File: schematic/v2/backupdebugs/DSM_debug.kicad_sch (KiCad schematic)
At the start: 16 parts, among them J16 DSM_DBG, J20 USB_A, U33 CH340G, Y2 Crystal

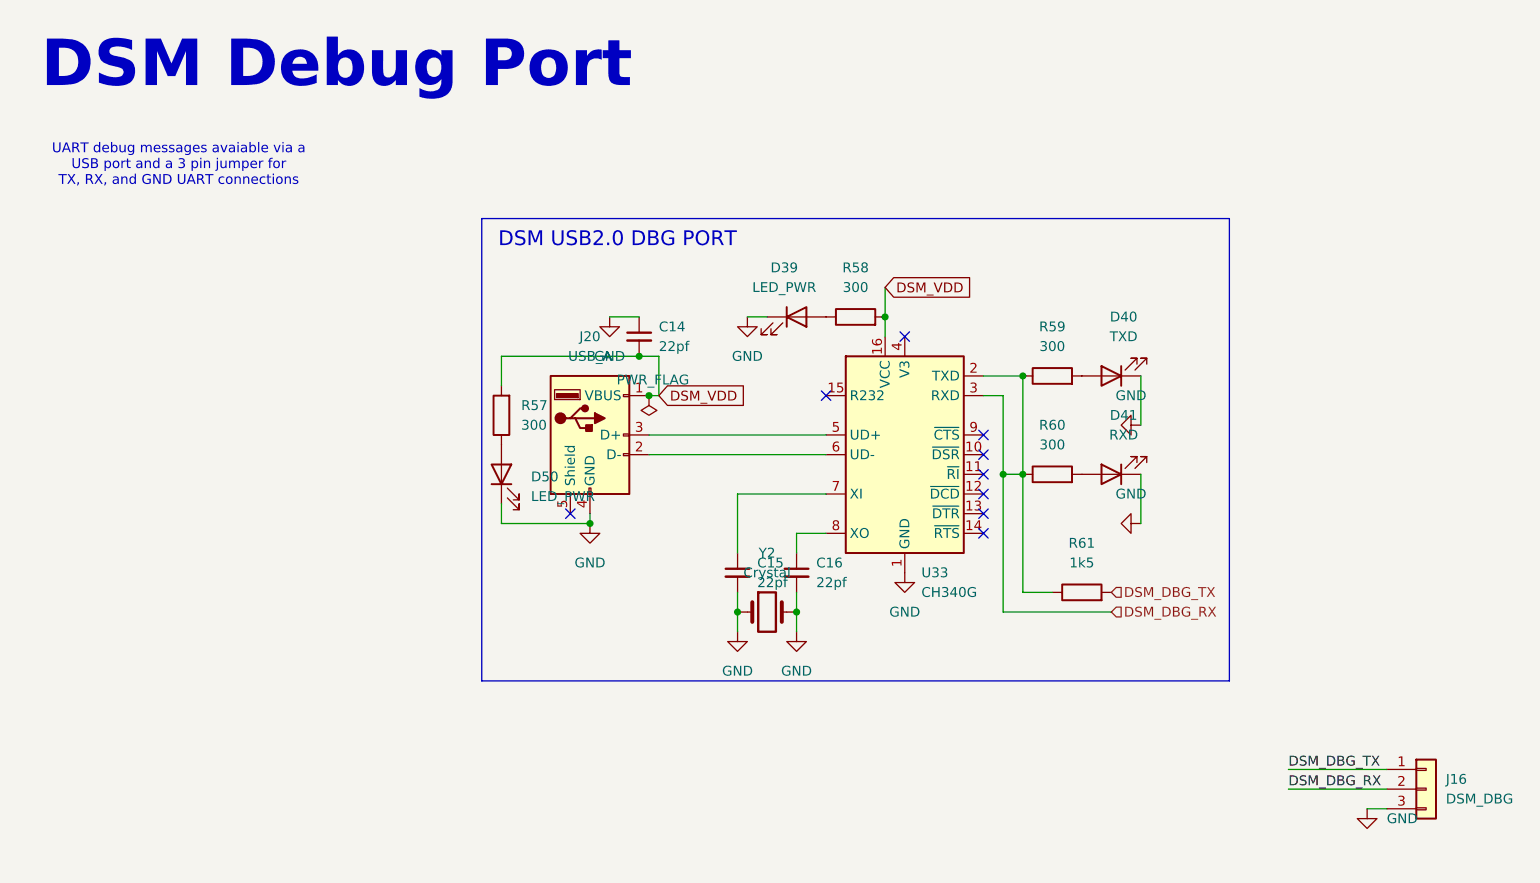
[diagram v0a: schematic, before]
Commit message: time to start routing?
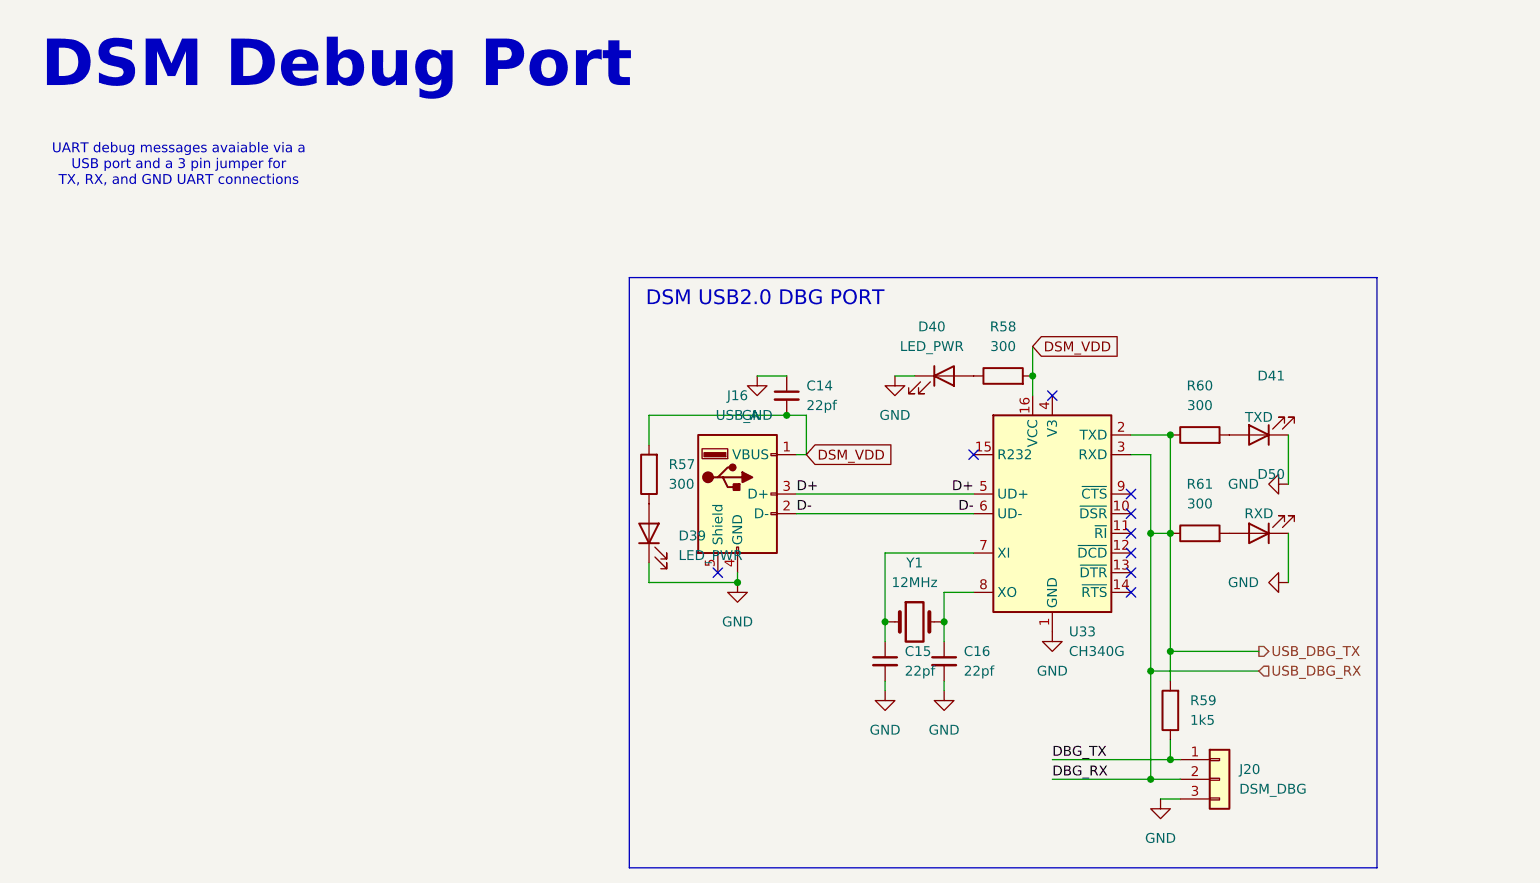
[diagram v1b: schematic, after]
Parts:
- removed J16: DSM_DBG, Connector_PinHeader_1.00mm:PinHeader_1x03_P1.00mm_Horizontal, symbol Connector_Generic:Conn_01x03
- removed J20: USB_A, Connector_USB:USB_A_CNCTech_1001-011-01101_Horizontal, symbol Connector:USB_A
- removed Y2: Crystal, symbol Device:Crystal
- added J16: USB_A, Connector_USB:USB_A_CNCTech_1001-011-01101_Horizontal, symbol Connector:USB_A
- added J20: DSM_DBG, Connector_PinHeader_1.00mm:PinHeader_1x03_P1.00mm_Horizontal, symbol Connector_Generic:Conn_01x03
- added Y1: 12MHz, Crystal:Crystal_HC49-4H_Vertical, symbol Device:Crystal
- D40: value TXD -> LED_PWR
- D41: value RXD -> TXD
- D50: value LED_PWR -> RXD
- R59: value 300 -> 1k5
- R61: value 1k5 -> 300
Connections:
- net DSM_VDD: now also J16.1 (VBUS)
- net GND: now also J16.4 (GND), J20.3 (Pin_3)
- net at R57.1: now also D39.2 (A); no longer D50.2 (A)
- net D+: now reaches U33.5 (UD+)
- net D+: now also J16.3 (D+)
- net D-: now reaches U33.6 (UD-)
- net D-: now also J16.2 (D-)
- net at C15.1, U33.7 (XI): now also Y1.1
- net at C16.1, U33.8 (XO): now also Y1.2
- net at D40.2 (A): now also R58.1; no longer R59.2
- net DSM_DBG_RX renamed USB_DBG_RX
- net USB_DBG_RX: now also R59.2, J20.2 (Pin_2); no longer R59.1
- net DSM_DBG_TX: no longer names the net of R61.2
- net DSM_DBG_TX: now also D50.2 (A)
- new net DBG_TX: J20.1 (Pin_1), R59.1
